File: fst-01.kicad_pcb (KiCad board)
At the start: 2 copper layers, 26.5 x 13.1 mm, 25 parts, among them J1 USB_A, K1 CONN_3, K2 CONN_2, K3 CONN_2, U1 STM32F103TB, U2 LP2985-33DBVR, U3 NUF2221W1, U4 SST25VF032B, X1 12MHz

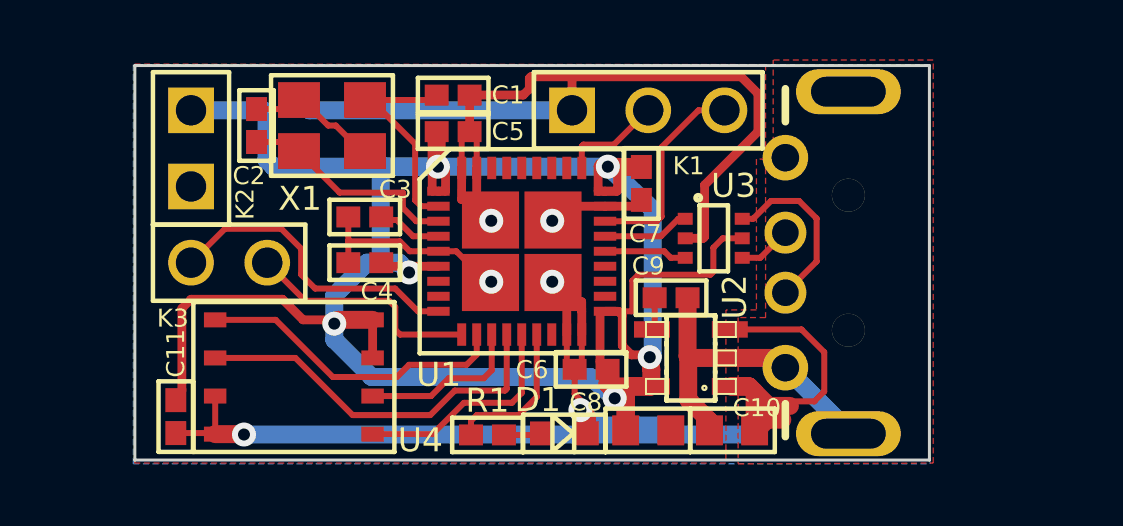
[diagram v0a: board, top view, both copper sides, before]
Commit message: added & improved FST-01R design
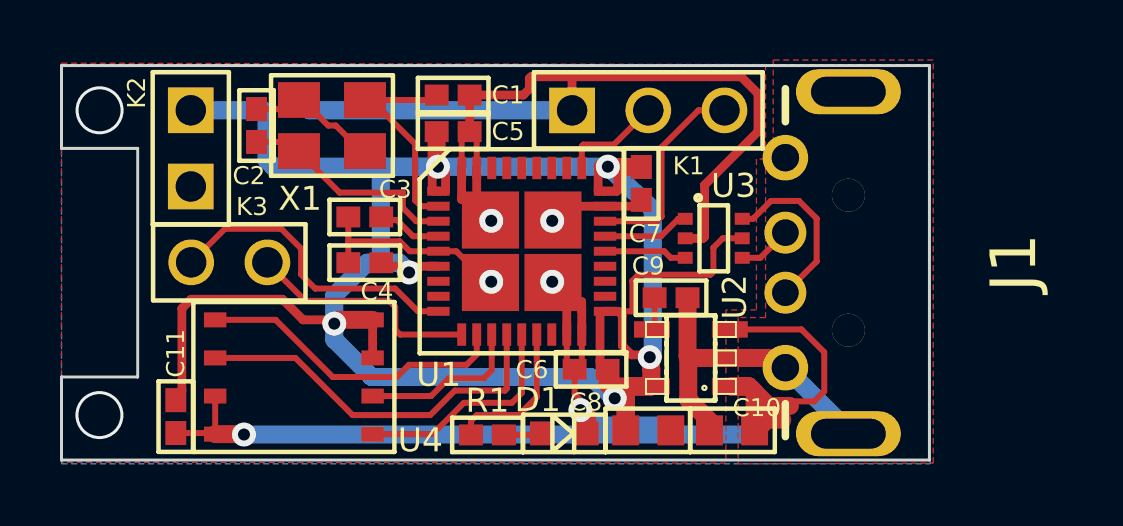
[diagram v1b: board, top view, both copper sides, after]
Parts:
- removed CE_mark: Symbol_CE_SilkScreen_5mm, Symbols:Symbol_CE_SilkScreen_5mm
- removed FST-LOGO: VAL**, FST-LOGO
- removed REF***: WEEE-Logo_4.2x6mm_SilkScreen, FST:WEEE-Logo_4.2x6mm_SilkScreen
- K1: value CONN_3 -> K1; footprint SIL-3-2 -> FST:SIL-3-2
- K2: value CONN_2 -> K2; footprint SIL-2-0 -> FST:SIL-2-0
- K3: value CONN_2 -> K3; footprint SIL-2-2 -> FST:SIL-2-2
- U1: value STM32F103TB -> GD32F103TB
- U3: footprint SOT363 -> FST:SOT363
- U4: footprint WSON8 -> FST:WSON8
- turned K3 to 180 degrees
- turned K2 to 90 degrees
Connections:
- K2 pad 1: +3V3 -> GND
- K2 pad 2: GND -> +3V3
- K3 pad 1: /PA2 -> /PA3
- K3 pad 2: /PA3 -> /PA2
- U1 pad 16: (no net) -> Net-(U1-Pad16)
- U1 pad 20: (no net) -> Net-(U1-Pad20)
- U1 pad 21: (no net) -> Net-(U1-Pad21)
- U1 pad 22: (no net) -> Net-(U1-Pad22)
- U1 pad 29: (no net) -> Net-(U1-Pad29)
- U1 pad 30: (no net) -> Net-(U1-Pad30)
- U1 pad 31: (no net) -> Net-(U1-Pad31)
- U1 pad 32: (no net) -> Net-(U1-Pad32)
- U1 pad 33: (no net) -> Net-(U1-Pad33)
- U1 pad 34: (no net) -> Net-(U1-Pad34)
- U1 pad 7: (no net) -> Net-(U1-Pad7)
- U1 pad 8: (no net) -> Net-(U1-Pad8)
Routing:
- net GND: vias 6 -> 8
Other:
- board size 26.5 x 13.1 mm -> 28.9 x 13.1 mm
